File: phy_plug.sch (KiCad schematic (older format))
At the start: 18 parts, among them J6 HY951180A_RJ45, U1 KSZ8081

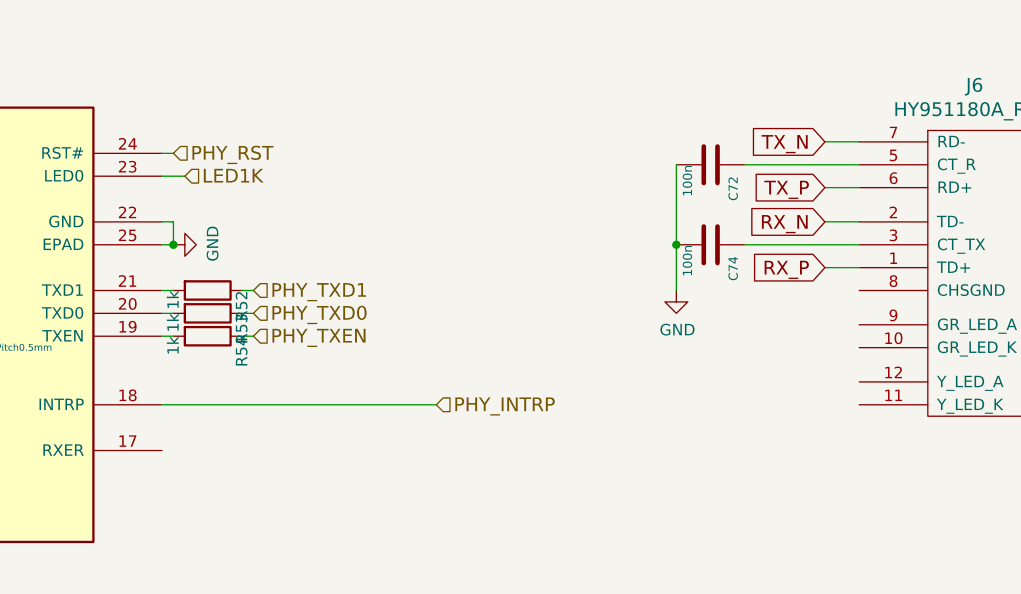
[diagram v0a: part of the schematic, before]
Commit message: V2 hardware
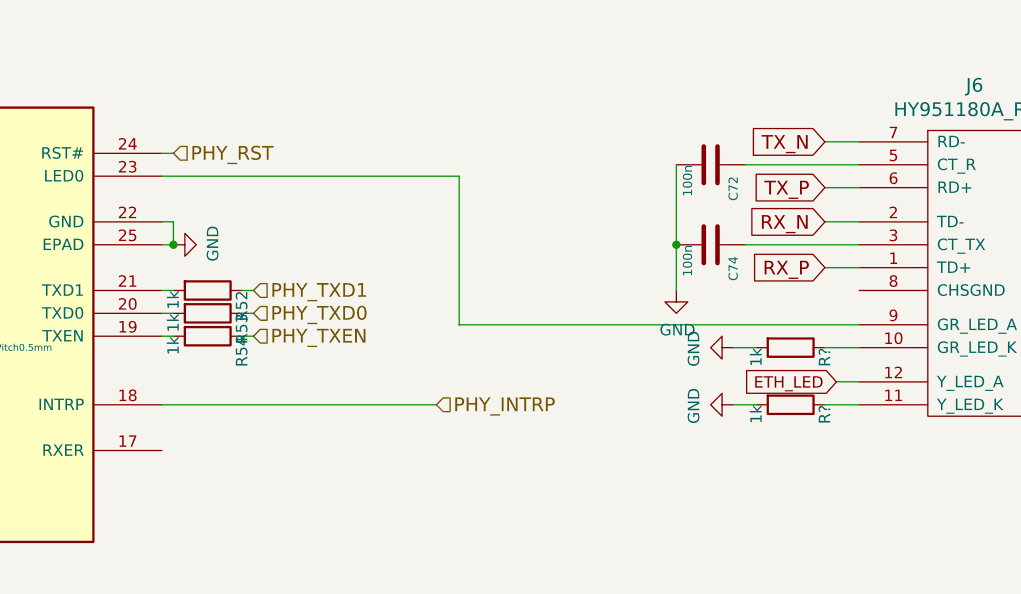
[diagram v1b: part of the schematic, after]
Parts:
- added R? (x2): 1k, stmbl:R_0603, symbol stmbl:R
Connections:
- net LED1K is gone; now on an unnamed net: U1.23 (LED0)
- net GND: now also R?.2, R?.2
- net at J6.10 (GR_LED_K): now also R?.1
- net at J6.11 (Y_LED_K): now also R?.1
- net ETH_LED: now reaches J6.12 (Y_LED_A)
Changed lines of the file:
@@
 Wire Wire Line
 	3400 5700 3400 5850
-Text HLabel 4500 3800 2    60   Input ~ 0
-LED1K
-Wire Wire Line
-	4400 3800 4500 3800
 Text HLabel 4450 3700 2    60   Input ~ 0
 PHY_RST
@@
 	1    0    0    -1
 $EndComp
+Wire Wire Line
+	7300 4550 7450 4550
+$Comp
+L stmbl:R R?
+U 1 1 5D4500D6
+P 7150 4550
+F 0 "R?" H 7150 4700 50  0000 L CNN
+F 1 "1k" H 7150 4400 50  0000 L CNN
+F 2 "stmbl:R_0603" V 7080 4550 50  0001 C CNN
+F 3 "" H 7150 4550 50  0000 C CNN
+	1    7150 4550
+	0    1    1    0
+$EndComp
+$Comp
+L power:GND #PWR?
+U 1 1 5D4518CE
+P 6900 4550
+F 0 "#PWR?" H 6900 4300 50  0001 C CNN
+F 1 "GND" H 6905 4377 50  0000 C CNN
+F 2 "" H 6900 4550 50  0000 C CNN
+F 3 "" H 6900 4550 50  0000 C CNN
+	1    6900 4550
+	0    1    1    0
+$EndComp
+Wire Wire Line
+	6900 4550 7000 4550
+$Comp
+L stmbl:R R?
+U 1 1 5D454373
+P 7150 4800
+F 0 "R?" H 7150 4950 50  0000 L CNN
+F 1 "1k" H 7150 4650 50  0000 L CNN
+F 2 "stmbl:R_0603" V 7080 4800 50  0001 C CNN
+F 3 "" H 7150 4800 50  0000 C CNN
+	1    7150 4800
+	0    1    1    0
+$EndComp
+Wire Wire Line
+	7300 4800 7450 4800
+$Comp
+L power:GND #PWR?
+U 1 1 5D45437E
+P 6900 4800
+F 0 "#PWR?" H 6900 4550 50  0001 C CNN
+F 1 "GND" H 6905 4627 50  0000 C CNN
+F 2 "" H 6900 4800 50  0000 C CNN
+F 3 "" H 6900 4800 50  0000 C CNN
+	1    6900 4800
+	0    1    1    0
+$EndComp
+Wire Wire Line
+	6900 4800 7000 4800
+Wire Wire Line
+	5700 4450 5700 3800
+Wire Wire Line
+	4400 3800 5700 3800
+Wire Wire Line
+	5700 4450 7450 4450
+Wire Wire Line
+	7350 4700 7450 4700
+Text GLabel 7350 4700 0    50   Input ~ 0
+ETH_LED
 $EndSCHEMATC
